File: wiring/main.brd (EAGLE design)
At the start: 98.7 x 76.2 mm, 38 parts, among them IC1 attiny 2313A, J2 J7MM, J3 J5MM, J4 J10MM, J5 J7MM, J6 J5MM, J7 J5MM, Q1 12MHz, T1 BD433, X1 USB-B

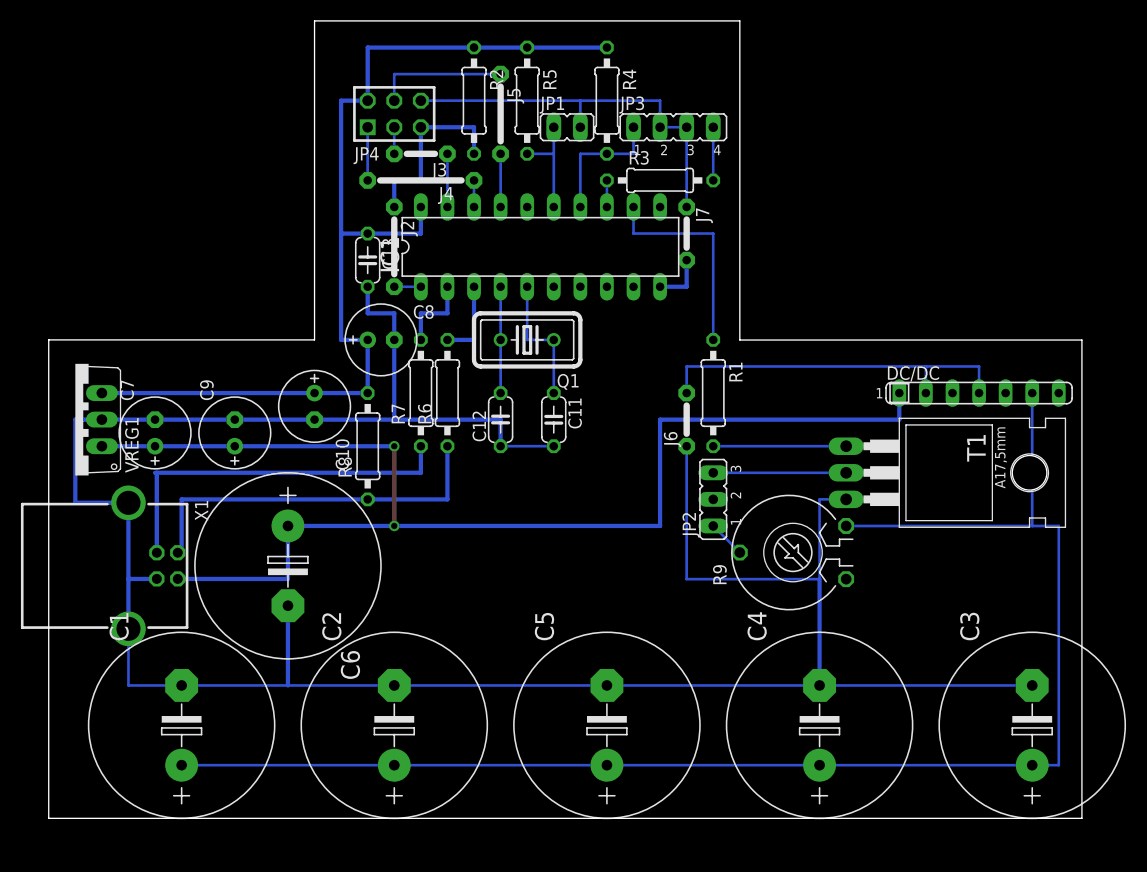
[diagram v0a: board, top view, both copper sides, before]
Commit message: ändern auf mosfet
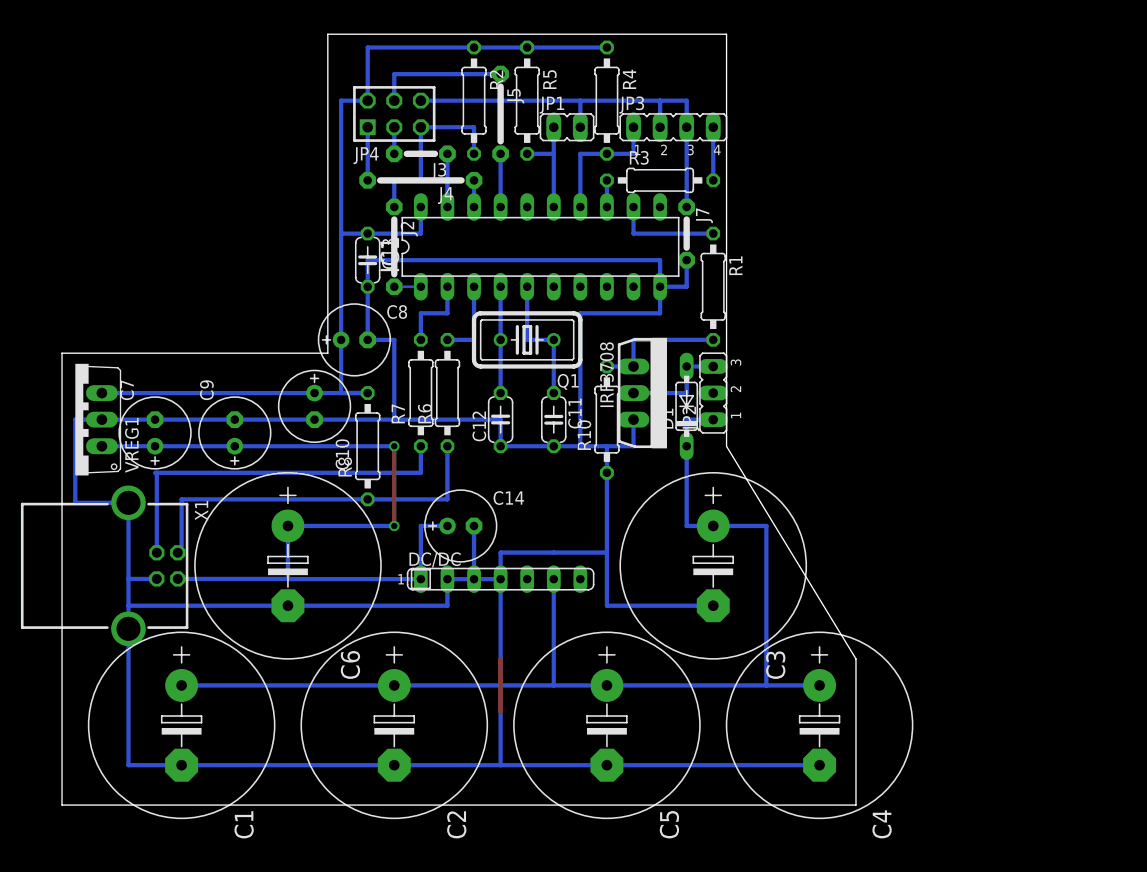
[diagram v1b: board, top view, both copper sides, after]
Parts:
- removed J6: J5MM, jumper:05
- removed R9: 1k, pot:PT-10
- removed T1: BD433, transistor:TO220
- added C14: 220µ, resistor:E2,5-7
- added D1: 1N4148DO35-7, diode:DO35-7
- added IRF3708: IRF3704L-V, transistor-power:TO262-V
- added R10: 10k, rcl:0207/10
- R1: value 1k -> 100
- moved DC/DC 49.1 mm to (43.2, 22.9)
- moved C3 34.1 mm to (63.5, 24.1), turned to 270 degrees
- moved JP2 10.2 mm to (63.5, 40.6)
- moved R1 10.2 mm to (63.5, 50.8)
- moved C8 2.54 mm to (29.2, 45.7)
- turned C1 to 270 degrees
- turned C2 to 270 degrees
- turned C4 to 270 degrees
- turned C5 to 270 degrees
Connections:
- removed net N$21: DC/DC.2, DC/DC.4, J6.2
- removed net N$5: JP2.1, R9.S
- net 5V: now also C14.+
- net GND: now also C14.-, DC/DC.2, DC/DC.4, IRF3708.3, R10.1; no longer J6.1, T1.3
- net N$2: now also IRF3708.1, R10.2; no longer T1.1
- net N$3: now also D1.A, IRF3708.2; no longer T1.2
- net N$4: now also D1.C, JP2.1; no longer R9.E
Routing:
- net GND: track 241.5 -> 340.5 mm
- net 5V: track 122.3 -> 81.6 mm
- net N$21: track 35.6 -> 0.00 mm
- net N$4: track 139.7 -> 106.7 mm
- net N$1: track 20.3 -> 10.2 mm
- net N$5: track 3.59 -> 0.00 mm
- net N$3: track 12.7 -> 10.2 mm
- net N$22: track 38.1 -> 40.6 mm
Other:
- board size 98.7 x 76.2 mm -> 75.9 x 73.7 mm
